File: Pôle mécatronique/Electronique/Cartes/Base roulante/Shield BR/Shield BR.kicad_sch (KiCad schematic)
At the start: 21 parts, among them J0 Conn_01x04_Female, J1 Conn_01x04_Female, J2 Conn_01x04_Female, J3 Conn_01x04_Female, J4 Conn_01x04_Male, J5-CAN1 Conn_01x02_Female, SW2 SW_Push_SPDT, U1 MCP2551-I-P, U4 R-78E5.0-0.5

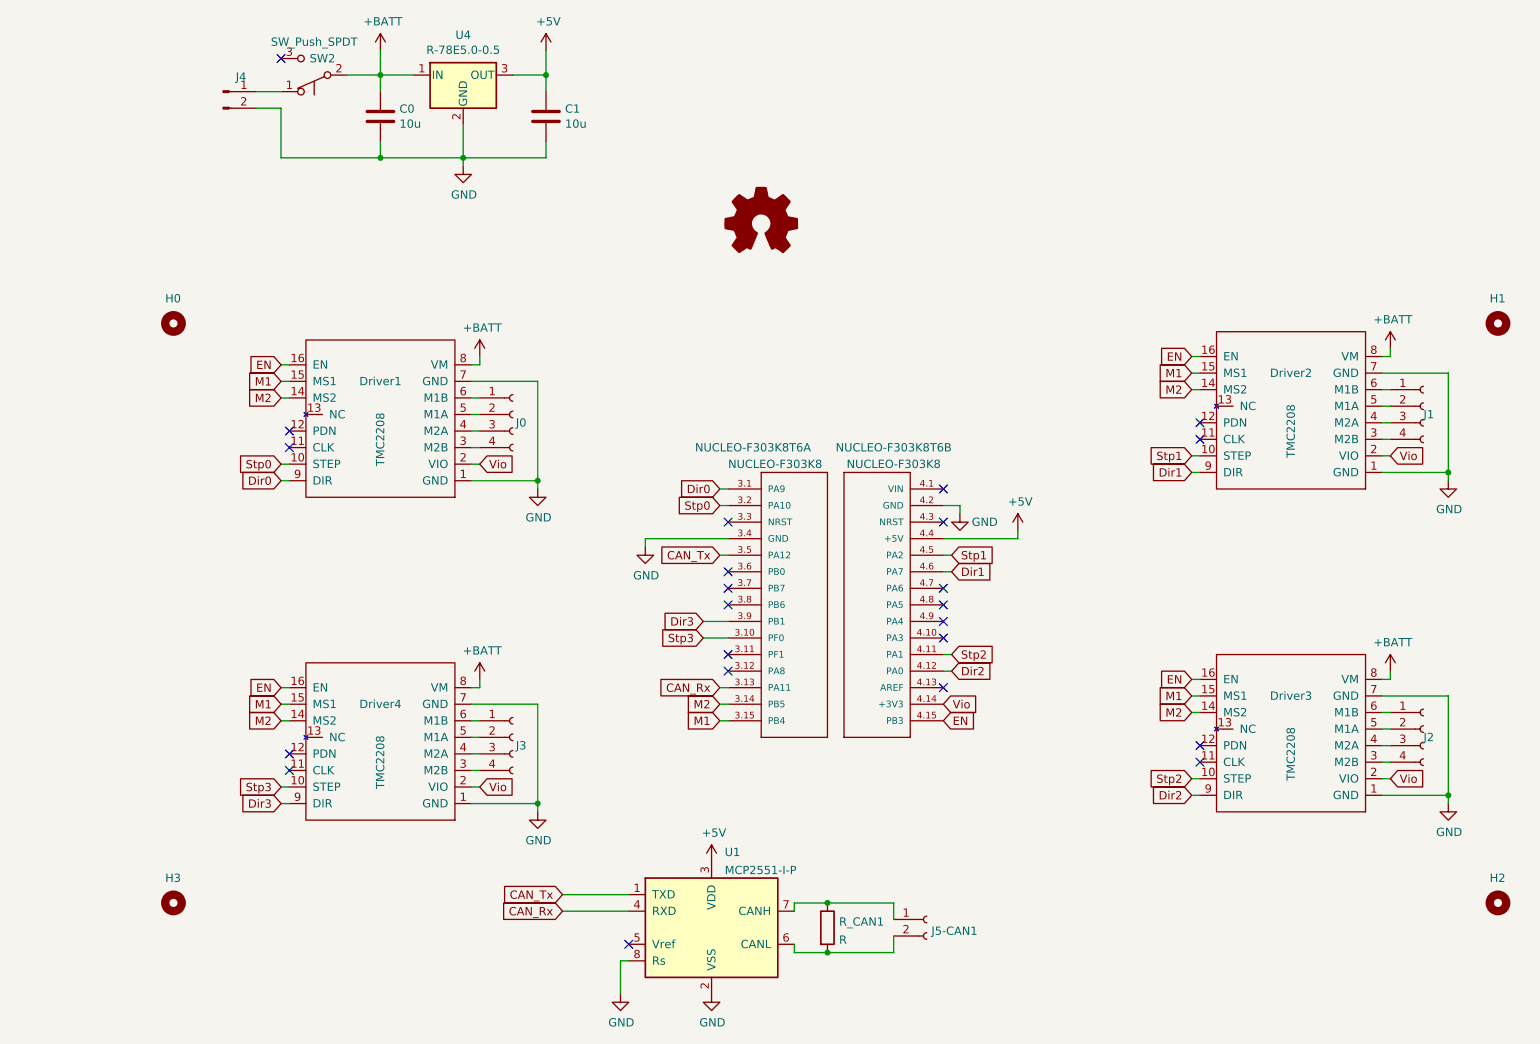
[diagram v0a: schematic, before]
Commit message: Update BR
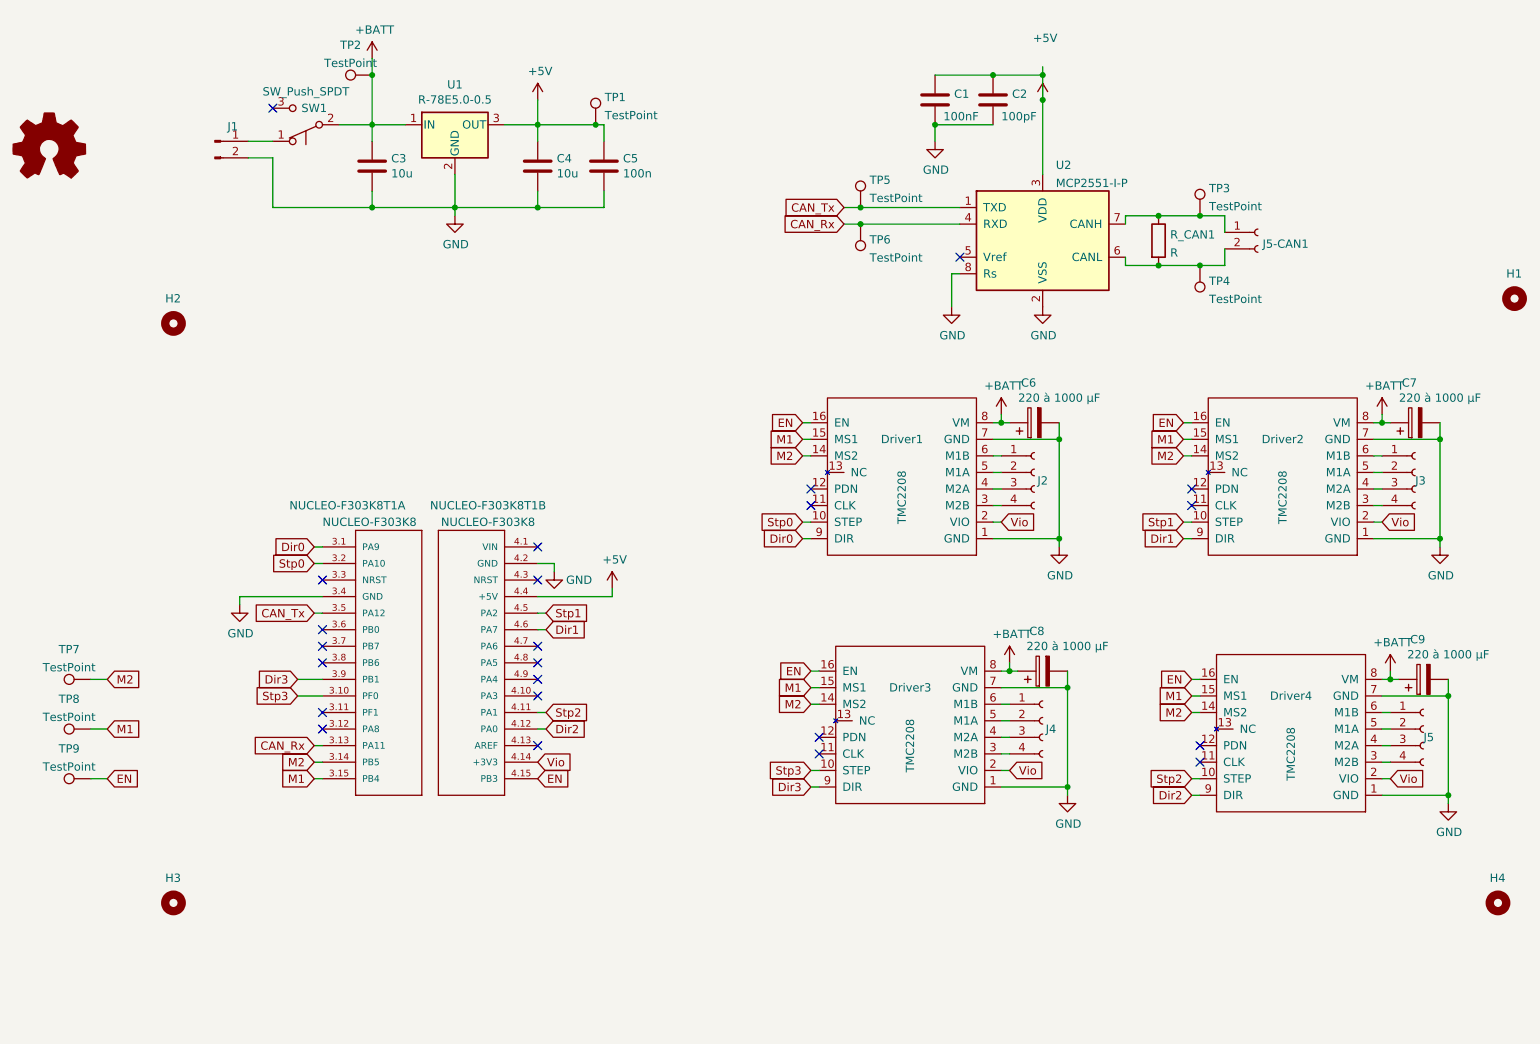
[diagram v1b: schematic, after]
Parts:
- added C1: 100nF, Capacitor_SMD:C_1206_3216Metric_Pad1.33x1.80mm_HandSolder, symbol Device:C
- added C2: 100pF, Capacitor_SMD:C_1206_3216Metric_Pad1.33x1.80mm_HandSolder, symbol Device:C
- added C5: 100n, Capacitor_SMD:C_1206_3216Metric_Pad1.33x1.80mm_HandSolder, symbol Device:C
- added C6, C7, C8, C9: 220 à 1000 µF, Capacitor_SMD:C_Elec_8x10.2, symbol Device:C_Polarized
- added TP1, TP2, TP3, TP4, TP5, TP6, TP7, TP8, TP9: TestPoint, TestPoint:TestPoint_Pad_D2.0mm, symbol Connector:TestPoint
- C3: renamed from C0; footprint Capacitor_SMD:C_1206_3216Metric_Pad1.42x1.75mm_HandSolder -> Capacitor_SMD:C_1206_3216Metric_Pad1.33x1.80mm_HandSolder
- C4: renamed from C1; footprint Capacitor_SMD:C_1206_3216Metric_Pad1.42x1.75mm_HandSolder -> Capacitor_SMD:C_1206_3216Metric_Pad1.33x1.80mm_HandSolder
- renumbered Driver4 to Driver3, Driver3 to Driver4, H0 to H2, H2 to H4, J4 to J1, J0 to J2, J1 to J3, J3 to J4, J2 to J5, NUCLEO-F303K8T6 to NUCLEO-F303K8T1, SW2 to SW1, U4 to U1, U1 to U2
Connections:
- net +5V: now also C1.1, C2.1, C5.1, TP1.1
- net +BATT: now also C6.1, C7.1, C8.1, C9.1, TP2.1
- net CAN_Rx: now also TP6.1
- net CAN_Tx: now also TP5.1
- net EN: now also TP9.1
- net GND: now also C1.2, C2.2, C5.2, C6.2, C7.2, C8.2, C9.2
- net M1: now also TP8.1
- net M2: now also TP7.1
- net at J5-CAN1.1 (Pin_1), R_CAN1.1, U2.7 (CANH): now also TP3.1
- net at J5-CAN1.2 (Pin_2), R_CAN1.2, U2.6 (CANL): now also TP4.1
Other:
- moved on the sheet: C3, C4, Driver1, Driver2, Driver3, H1, J1, J2, J3, J4, J5-CAN1, NUCLEO-F303K8T1A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
